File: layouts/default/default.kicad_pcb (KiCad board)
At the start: 4 copper layers, 27.5 x 14.2 mm, 17 parts

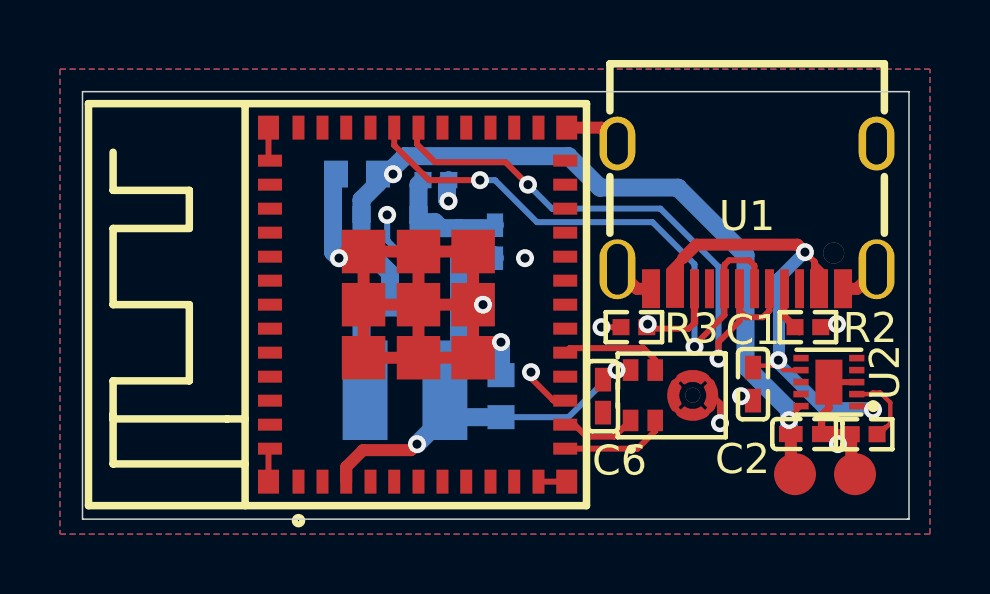
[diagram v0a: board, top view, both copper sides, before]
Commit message: eod
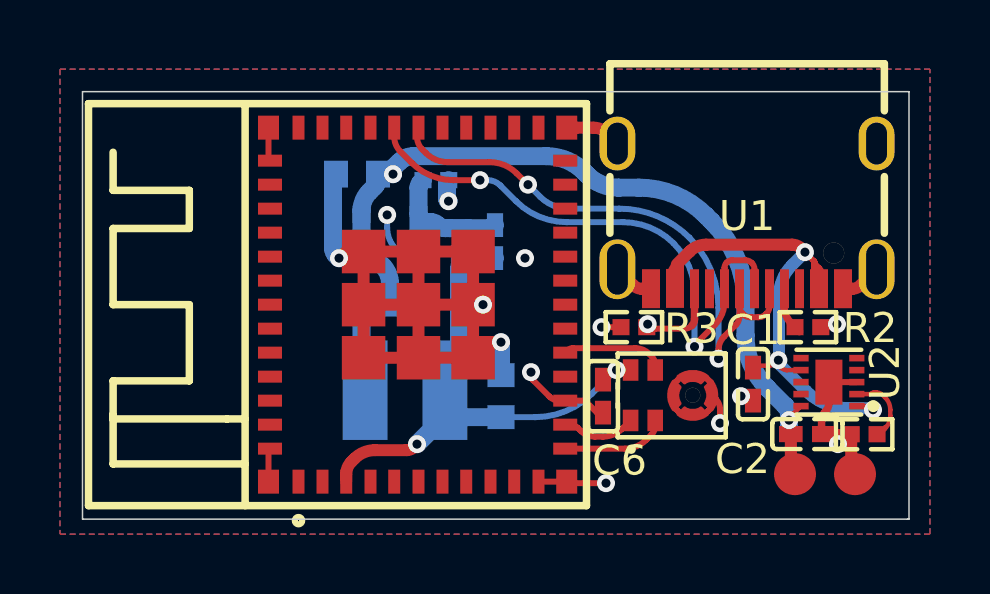
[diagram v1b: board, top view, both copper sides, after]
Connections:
- net B5 renamed CC2
- net B8 renamed SUB2
- net CC1 renamed A5
- net SUB1 renamed A8
- C2 pad 1: hv -> hv-2
- C3 pad 1: hv-2 -> hv
- C4 pad 1: hv -> hv-2
- C5 pad 1: hv-2 -> hv
- C6 pad 1: hv-2 -> hv
- L1 pad 18: uc-line-2 -> uc-line-7
- L1 pad 22: uc-line-11 -> uc-line-8
- L1 pad 23: uc-line-3 -> uc-line-9
- L1 pad 24: uc-line -> uc-line-12
- L1 pad 26: uc-line-1 -> uc-line-5
- L1 pad 27: uc-line-7 -> uc-line-4
- L1 pad 28: uc-line-13 -> uc-line-11
- L1 pad 29: uc-line-12 -> uc-line-1
- L1 pad 3: hv-2 -> hv
- L1 pad 32: uc-line-9 -> uc-line
- L1 pad 33: uc-line-4 -> uc-line-2
- L1 pad 5: uc-line-5 -> uc-line-3
- L1 pad 6: uc-line-8 -> uc-line-10
- L1 pad 8: uc-line-10 -> EN
- L2 pad 2: hv-2 -> hv
- MIC1 pad 5: hv-2 -> hv
- R5 pad 1: hv-2 -> hv
- U2 pad 10: hv -> hv-2
- U3 pad 4: hv -> hv-2
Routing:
- net hv: track 25.0 -> 19.3 mm
- net hv-2: track 19.9 -> 24.1 mm
- net gnd: track 52.2 -> 55.7 mm, vias 11 -> 12
- net line-1: track 20.0 -> 19.4 mm
- net hv-1: track 20.3 -> 19.7 mm
- net EN: track 3.27 -> 3.17 mm, vias 1 -> 0
- net (no net): vias 0 -> 1
